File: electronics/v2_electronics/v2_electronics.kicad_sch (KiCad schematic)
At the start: 30 parts, among them J1 Main Connector, J2 Main Power, J3 12-6V Converter, J4 Battery Connector, J5 Depth Sensor, K1 G5Q-1, K2 G5Q-1, K3 G5Q-1, K4 G5Q-1, Q1 BC547, Q2 BC547, Q3 BC547, Q4 BC547, Q8 BC547, U1 raspberry_pi_pico, U2 mpu6050_breakout

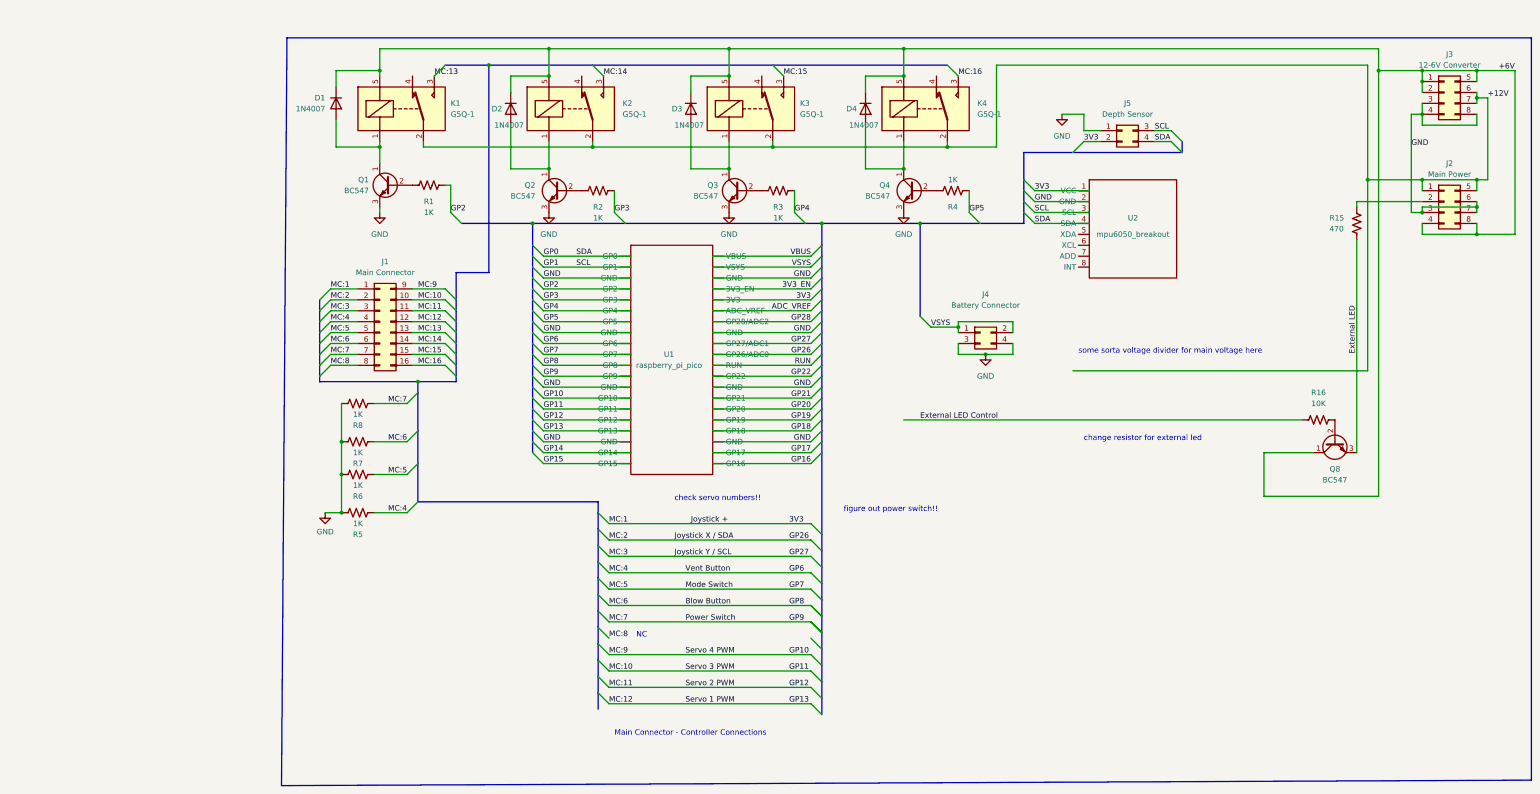
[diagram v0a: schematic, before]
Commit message: more pcb v2 work:
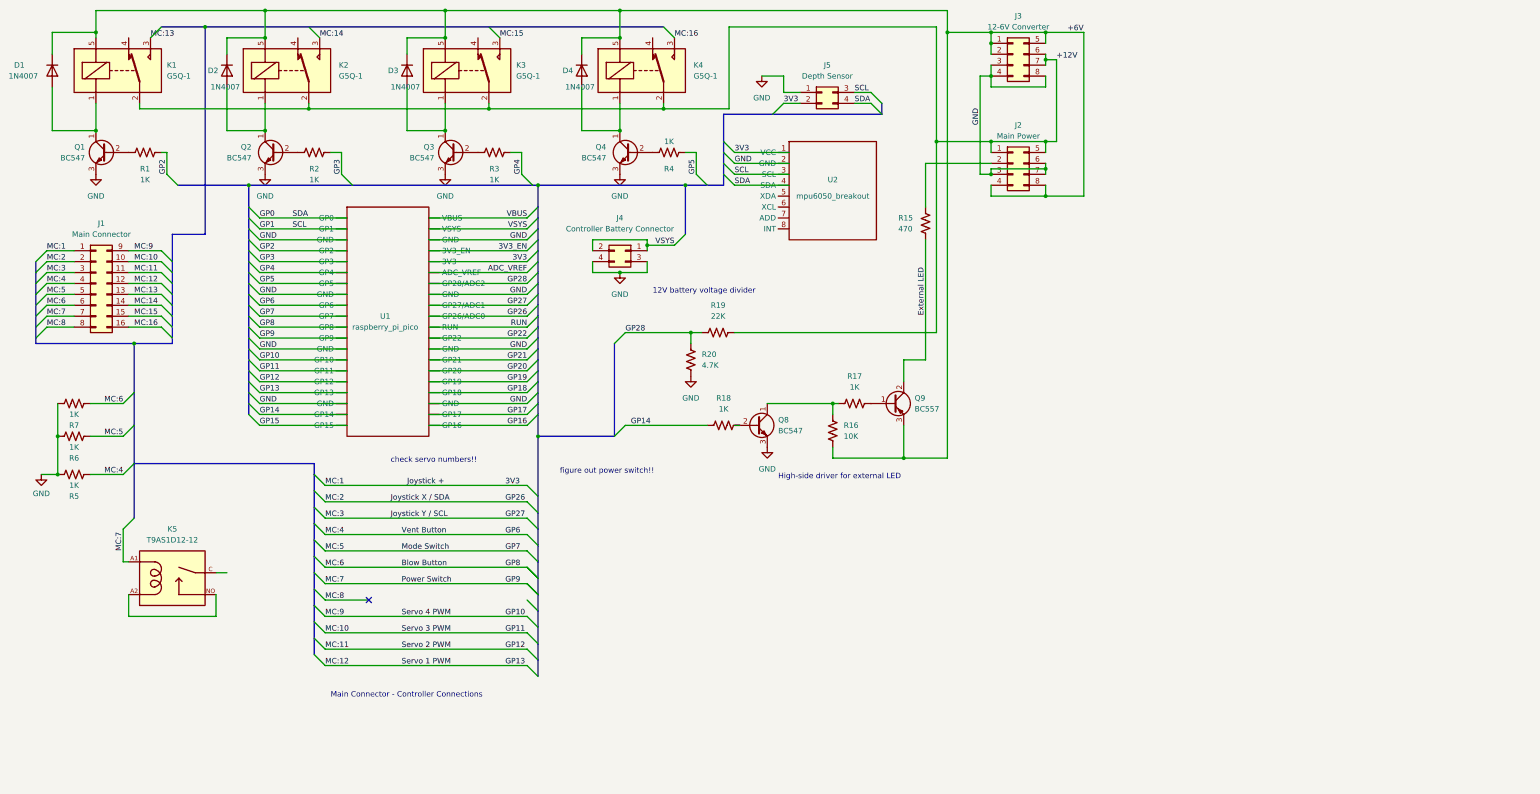
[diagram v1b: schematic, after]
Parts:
- removed R8: 1K, Resistor_THT:R_Axial_DIN0207_L6.3mm_D2.5mm_P10.16mm_Horizontal, symbol Device:R_US
- added K5: T9AS1D12-12, TE_1-1393210-3, symbol custom_parts:T9AS1D12
- added Q9: BC557, symbol Device:Q_PNP_BCE
- added R17, R18: 1K, Resistor_THT:R_Axial_DIN0207_L6.3mm_D2.5mm_P10.16mm_Horizontal, symbol Device:R_US
- added R19: 22K, Resistor_THT:R_Axial_DIN0207_L6.3mm_D2.5mm_P10.16mm_Horizontal, symbol Device:R_US
- added R20: 4.7K, Resistor_THT:R_Axial_DIN0207_L6.3mm_D2.5mm_P10.16mm_Horizontal, symbol Device:R_US
- J4: value Battery Connector -> Controller Battery Connector
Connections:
- net External LED Control is gone; now on net +6V: R16.1
- net +12V: now also R19.2
- net +6V: now also Q9.3 (E); no longer Q8.1 (C)
- net External LED: now also Q9.2 (C); no longer Q8.3 (E)
- net GND: now also Q8.3 (E), R20.1
- net GP14: now also R18.1
- net GP28: now also R19.1, R20.2
- net GP9: now also K5.A1
- net at R16.2: now also Q8.1 (C), R17.1; no longer Q8.2 (B)
- new net: Q8.2 (B), R18.2
- new net: Q9.1 (B), R17.2
- new net: K5.A2, K5.NO
- no-connect marks 0 -> 1
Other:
- note added: "12V battery voltage divider"
- note added: "High-side driver for external LED"
- note removed: "NC"
- note removed: "change resistor for external led"
- note removed: "some sorta voltage divider for main voltage here"
- moved on the sheet: D1, D2, D3, D4, J1, J2, J3, J4, J5, K1, K2, K3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

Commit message: more work on schematic v2
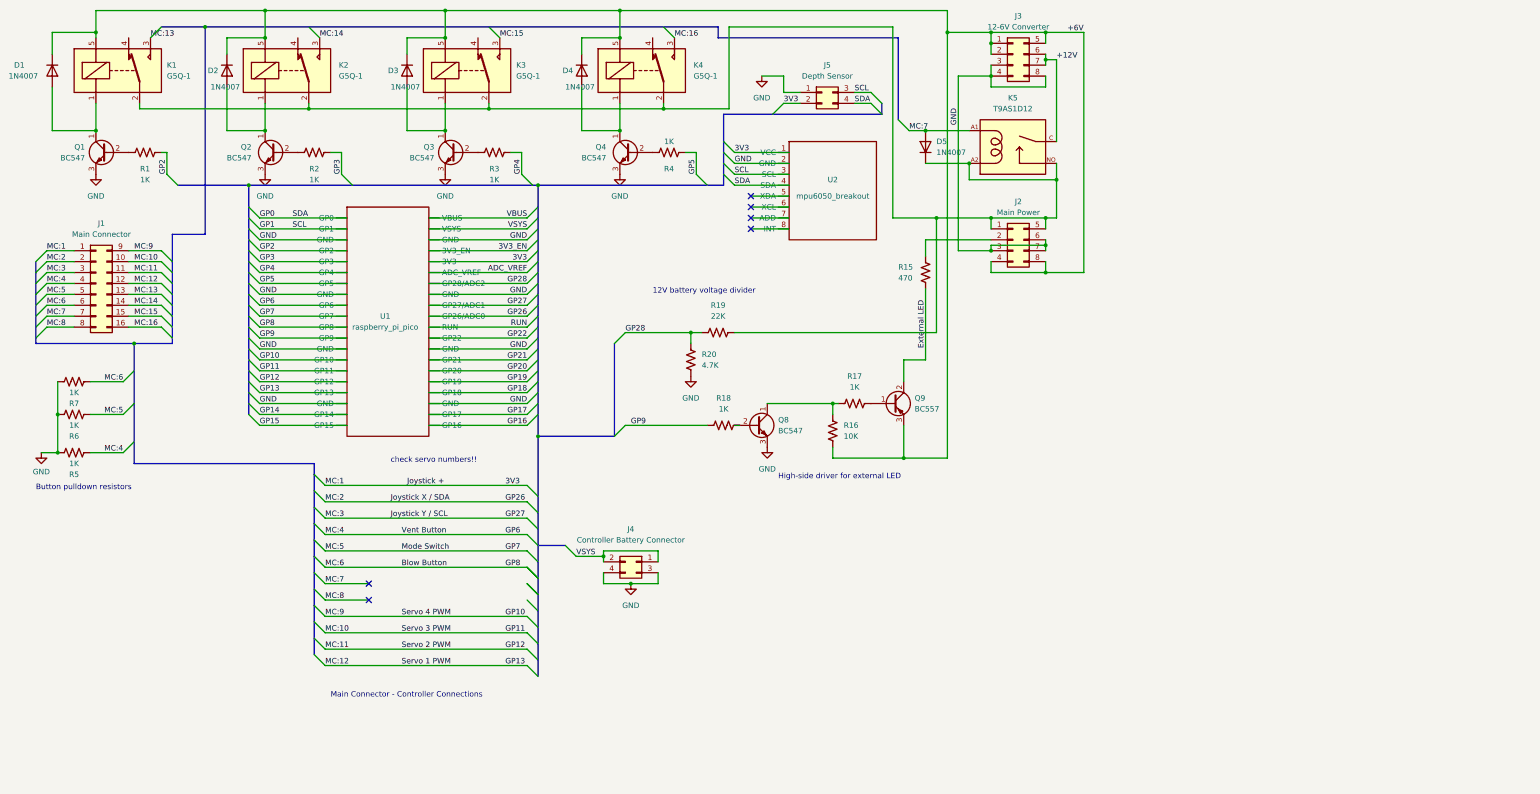
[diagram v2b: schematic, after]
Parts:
- added D5: 1N4007, Diode_THT:D_DO-41_SOD81_P10.16mm_Horizontal, symbol Diode:1N4007
- K5: value T9AS1D12-12 -> T9AS1D12; footprint TE_1-1393210-3 -> custom_footprints:T9AS1D12
- Q9: footprint (none) -> Package_TO_SOT_THT:TO-92_Inline
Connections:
- net +12V: now also K5.C; no longer J2.1 (Pin_1), J2.5 (Pin_5), K1.2, K2.2, K3.2, K4.2, R19.2
- net GP14: no longer R18.1
- net GP9: now also R18.1; no longer J1.7 (Pin_7), K5.A1
- net at K5.A2, K5.NO: now also J2.1 (Pin_1), J2.5 (Pin_5), K1.2, K2.2, K3.2, K4.2, R19.2, D5.1 (K)
- new net MC:7: D5.2 (A), J1.7 (Pin_7), K5.A1
- no-connect marks 1 -> 6
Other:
- note added: "Button pulldown resistors"
- note removed: "figure out power switch!!"
- moved on the sheet: J2, R15, R5, R6, R7
